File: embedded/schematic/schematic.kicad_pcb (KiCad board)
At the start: 12 copper layers, 71.1 x 30.5 mm, 10 parts

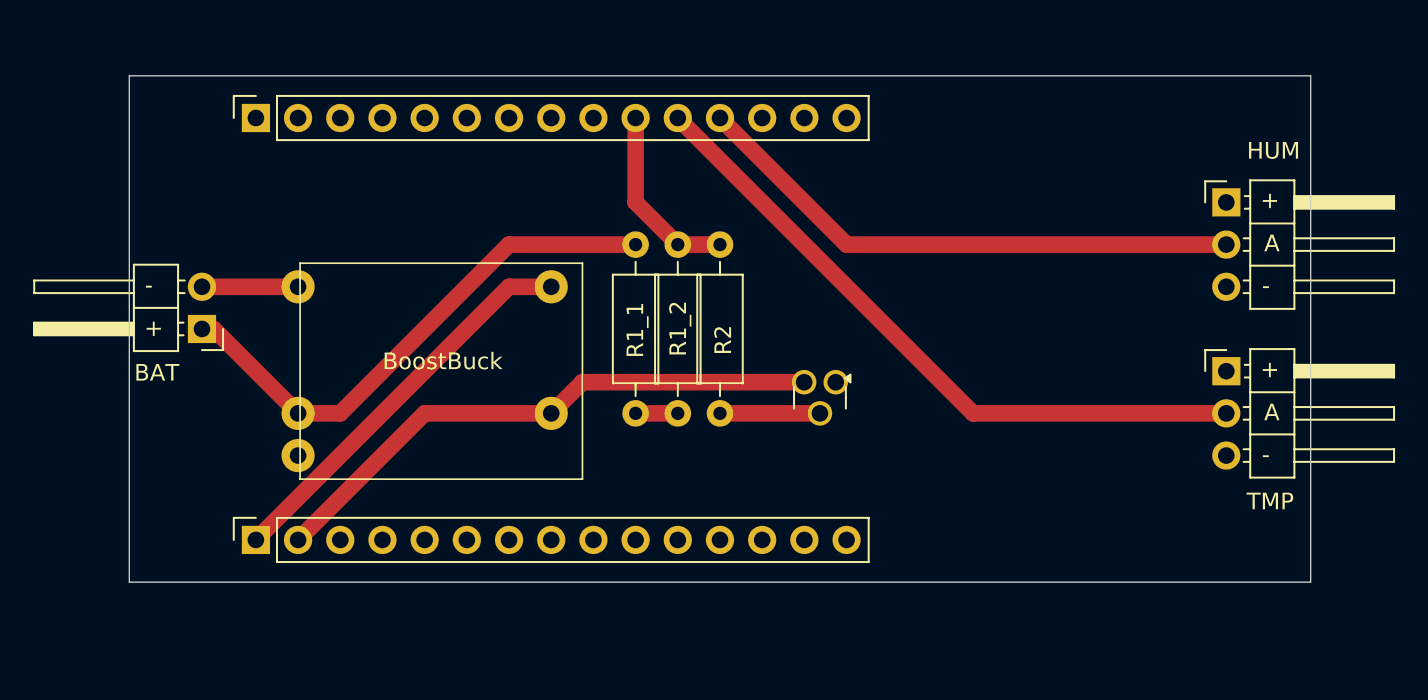
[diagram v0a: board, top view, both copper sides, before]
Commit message: Updated schematics
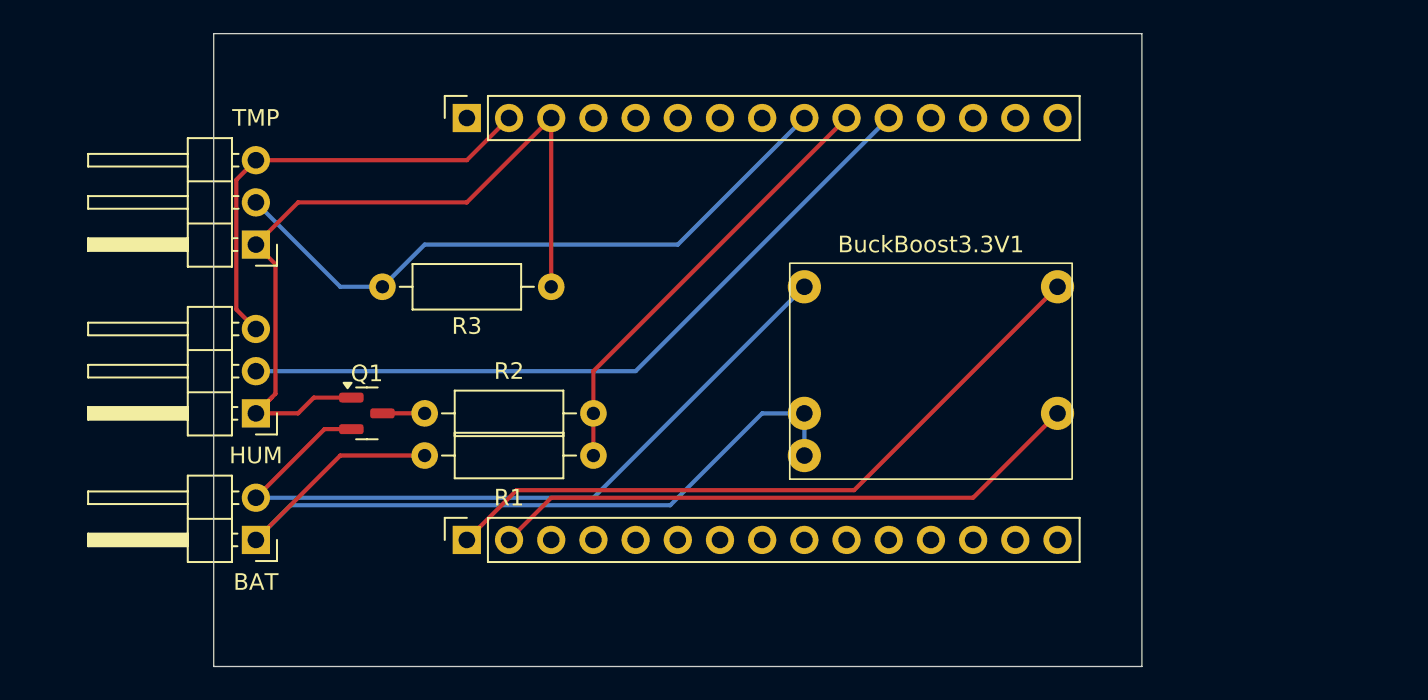
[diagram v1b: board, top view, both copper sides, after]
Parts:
- removed the REF** at (61.9, 47.3)
- removed the REF** at (86.4, 35.6)
- removed the REF** at (86.4, 45.7)
- removed the REF** at (53.3, 38.1)
- removed the REF** at (50.8, 38.1)
- removed the REF** at (55.9, 38.1)
- removed the REF** at (38.1, 45.7)
- removed the REF** at (24.7, 43.2)
- added BAT: PinHeader_1x02_P2.54mm_Horizontal, Connector_PinHeader_2.54mm:PinHeader_1x02_P2.54mm_Horizontal, F.Cu at (27.9, 55.9)
- added BuckBoost3.3V1: ~, custom:BuckBoost3.3V, F.Cu at (68.6, 45.7)
- added HUM: PinHeader_1x03_P2.54mm_Horizontal, Connector_PinHeader_2.54mm:PinHeader_1x03_P2.54mm_Horizontal, F.Cu at (27.9, 48.3)
- added Q1: AO3400A, Package_TO_SOT_SMD:SOT-23, F.Cu at (34.6, 48.3)
- added R1: 1M, Resistor_THT:R_Axial_DIN0207_L6.3mm_D2.5mm_P10.16mm_Horizontal, F.Cu at (38.1, 50.8)
- added R2: 1M, Resistor_THT:R_Axial_DIN0207_L6.3mm_D2.5mm_P10.16mm_Horizontal, F.Cu at (48.3, 48.3)
- added R3: 4.7k, Resistor_THT:R_Axial_DIN0207_L6.3mm_D2.5mm_P10.16mm_Horizontal, F.Cu at (45.7, 40.6)
- added TMP: PinHeader_1x03_P2.54mm_Horizontal, Connector_PinHeader_2.54mm:PinHeader_1x03_P2.54mm_Horizontal, F.Cu at (27.9, 38.1)
- moved REF** 28.4 mm to (40.6, 30.5)
- moved REF** 28.4 mm to (40.6, 55.9)
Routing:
- net (no net): track 330.1 -> 0.00 mm
- net GND: track 0.00 -> 109.3 mm
- net BAT+: track 0.00 -> 51.0 mm
- net SEN: track 0.00 -> 49.7 mm
- net HUM: track 0.00 -> 44.4 mm
- net 3.3V: track 0.00 -> 41.9 mm
- net TMP: track 0.00 -> 39.3 mm
- net BAT: track 0.00 -> 26.6 mm
- net Net-(Q1-D): track 0.00 -> 2.54 mm
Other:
- board size 71.1 x 30.5 mm -> 55.9 x 38.1 mm
- copper layers 12 -> 2
- board text removed: "+"
- board text removed: "-"
- board text removed: "A"
- board text removed: "BAT"
- board text removed: "BoostBuck"
- board text removed: "HUM"
- board text removed: "R1_1"
- board text removed: "R1_2"
- board text removed: "R2"
- board text removed: "TMP"
